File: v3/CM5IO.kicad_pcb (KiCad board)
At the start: 4 copper layers, 72 x 58 mm, 44 parts, among them J1 TYPE-C-31-M-12, J2 Conn_01x22_Female, J3 Conn_01x22_Female, J5 Conn_01x02, J6 UART Connection, J7 Micro_SD_Card_Det, J8 10164227-1001A1RLF, J9 10164227-1001A1RLF, Q1 AO3400A, SW1 Right angle Tact button, SW2 Right angle Tact button, U1 LSM9DS1, U2 74LVC1G07SE-7, U3 ASM330LHHTR, U4 XIAO_RM3100_Breakout, U5 RT9742GGJ5

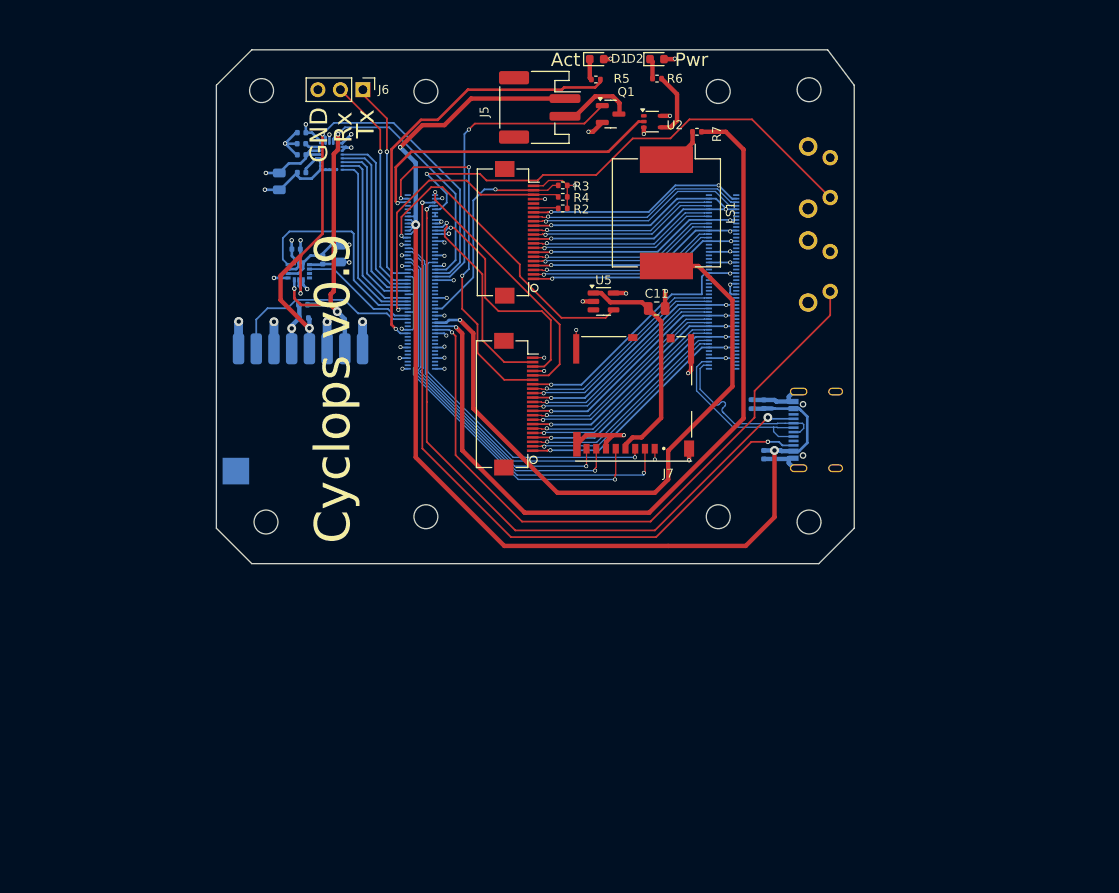
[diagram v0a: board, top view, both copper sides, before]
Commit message: Finalise v1.0 design
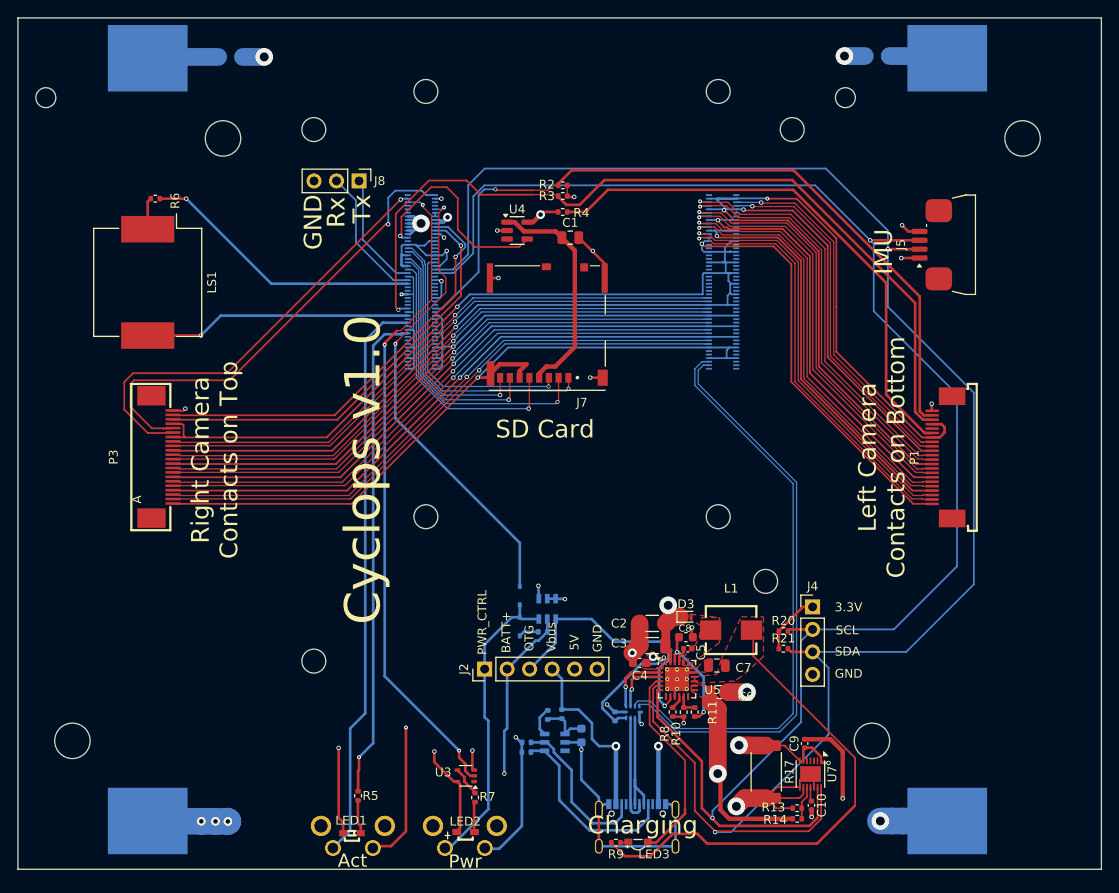
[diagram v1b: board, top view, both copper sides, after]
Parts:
- removed the C1 at (180.3, 111.7)
- removed D1: LED Green, LED_SMD:LED_0603_1608Metric
- removed D2: LED Red, LED_SMD:LED_0603_1608Metric
- removed the J3 at (152.4, 92.3)
- removed Q1: AO3400A, Package_TO_SOT_SMD:SOT-23
- removed the R4 at (157.6, 88.3)
- removed SW1, SW2: Right angle Tact button, Button_Switch_THT:SW_Tactile_SPST_Angled_PTS645Vx58-2LFS
- removed the U1 at (131.5, 83.7)
- removed the U3 at (127.8, 96.7)
- removed the U4 at (128.1, 112.2)
- added B1: BH-21700-B1BJ001, footprint:BAT-SMD_L82.5.5-W25-BH-21700-B1BJ001, B.Cu at (110.8, 115.7)
- added B2: BH-21700-B1BJ001, footprint:BAT-SMD_L82.5.5-W25-BH-21700-B1BJ001, B.Cu at (201.0, 115.7)
- added C11: 1uF, Capacitor_SMD:C_0603_1608Metric, B.Cu at (159.7, 149.1)
- added D3: NSR10F20NXT5G, Diode_SMD:Nexperia_DSN1608-2_1.6x0.8mm, F.Cu at (171.5, 135.7)
- added D5: D_Schottky, Diode_SMD:D_SOD-323, B.Cu at (152.8, 133.3)
- added D6: D_Schottky, Diode_SMD:D_SOD-323, B.Cu at (152.8, 136.8)
- added F1: Fuse, Fuse:Fuse_1206_3216Metric, B.Cu at (120.1, 72.5)
- added F2: Fuse, Fuse:Fuse_1206_3216Metric, B.Cu at (193.1, 72.4)
- added J4: Conn_01x04_Pin, Connector_PinHeader_2.54mm:PinHeader_1x04_P2.54mm_Vertical, F.Cu at (185.8, 134.6)
- added L1: MHCI05018-1R0M-R8A, footprint:IND-SMD_L5.7-W5.4, F.Cu at (176.6, 137.2)
- added LED1: MHS171CYCT, footprint:LED-SMD_L2.0-W1.1-R-RD-SIDE_YELLOW, F.Cu at (133.8, 160.1)
- added LED2: MHS171UGCT, footprint:LED-SMD_L2.0-W1.1_RD_GREEN_SIDE, F.Cu at (146.6, 160.0)
- added LED3: MHS171UBCT, footprint:LED-SMD_L2.1-W1.0-R-RD, F.Cu at (166.1, 161.1)
- added P1: AFC07-S22FCC-00 (Bottom contact), footprint:FPC-SMD_AFC07-S22FCC-00, F.Cu at (200.4, 117.7)
- added P3: FPC_0_5MM_22P_Pull_type_H2_0mm_Pick_up, footprint:FPC-SMD_P0.50-22P_LSSJ-H2.0-22P, F.Cu at (112.4, 117.7)
- added R10: 10k, Resistor_SMD:R_0402_1005Metric, F.Cu at (172.5, 146.4)
- added R11: 10k, Resistor_SMD:R_0402_1005Metric, F.Cu at (171.2, 146.5)
- added R12: 10k, Resistor_SMD:R_0402_1005Metric, B.Cu at (155.3, 137.4)
- added R13: 300k, Resistor_SMD:R_0402_1005Metric, F.Cu at (184.1, 158.5)
- added R14: 200k, Resistor_SMD:R_0402_1005Metric, F.Cu at (184.1, 157.3)
- added R15: 10k, Resistor_SMD:R_0402_1005Metric, B.Cu at (155.9, 146.8)
- added R16: 1k, Resistor_SMD:R_0402_1005Metric, B.Cu at (157.5, 146.7)
- added R17: 10mOhm, Resistor_SMD:R_2512_6332Metric, F.Cu at (180.6, 153.2)
- added R18: 5.1k, Resistor_SMD:R_0402_1005Metric, B.Cu at (153.5, 149.9)
- added R19: 5.1k, Resistor_SMD:R_0402_1005Metric, B.Cu at (153.5, 151.0)
- added R2: 2.2K 1%, Resistor_SMD:R_0402_1005Metric, F.Cu at (157.6, 87.0)
- added R20: 2.2K 1%, Resistor_SMD:R_0402_1005Metric, F.Cu at (182.5, 137.3)
- added R21: 2.2K 1%, Resistor_SMD:R_0402_1005Metric, F.Cu at (182.5, 139.3)
- added U10: TS-1093C-A5B3-D1, footprint:SW-TH_TS-1093C-A5B3-D1, B.Cu at (146.6, 160.5)
- added U2: TS3USB221ARSER, footprint:UQFN-10_L2.0-W1.5-P0.50-BL, B.Cu at (165.5, 146.4)
- added U5: BQ25895RTW, Package_DFN_QFN:Texas_RTW_WQFN-24-1EP_4x4mm_P0.5mm_EP2.7x2.7mm_ThermalVias, F.Cu at (170.5, 142.7)
- added U6: SN74LVC1G57DBVR, footprint:SOT-23-6_L2.9-W1.6-P0.95-LS2.8-BL, B.Cu at (155.8, 134.8)
- added U7: MAX17261xxTD, Package_DFN_QFN:TDFN-14-1EP_3x3mm_P0.4mm_EP1.78x2.35mm, F.Cu at (185.6, 153.4)
- added U8: CH221K, footprint:SOT-23-6_L2.9-W1.6-P0.95-LS2.8-BL-2, B.Cu at (156.7, 149.9)
- added U9: TS-1093C-A14B3-D1, footprint:SW-TH_TS-1093C-A14B3-D1, B.Cu at (133.9, 160.5)
- C1: renamed from C11; value 10u -> 10uF
- C10: value 10u -> 470nF; footprint Capacitor_SMD:C_0805_2012Metric -> Capacitor_SMD:C_0402_1005Metric; moved to F.Cu
- C2: value 100n -> 33uF; footprint Capacitor_SMD:C_0402_1005Metric -> Capacitor_SMD:C_1206_3216Metric; moved to F.Cu
- C3: value 10n -> 33uF; footprint Capacitor_SMD:C_0402_1005Metric -> Capacitor_SMD:C_1206_3216Metric; moved to F.Cu
- C4: value 100n -> 1uF; footprint Capacitor_SMD:C_0402_1005Metric -> Capacitor_SMD:C_0603_1608Metric; moved to F.Cu
- C5: value 100n -> 47nF; moved to F.Cu
- C6: value 10u -> 22uF; moved to F.Cu
- C7: value 100n -> 10uF; footprint Capacitor_SMD:C_0402_1005Metric -> Capacitor_SMD:C_0805_2012Metric; moved to F.Cu
- C8: value 100n -> 4.7uF; footprint Capacitor_SMD:C_0402_1005Metric -> Capacitor_SMD:C_0603_1608Metric; moved to F.Cu
- C9: value 100n -> 100nF; moved to F.Cu
- J2: value Conn_01x22_Female -> Conn_01x06_Pin; footprint CM5IO:Hirose_FH12-22S-0.5SH_1x22-1MP_P0.50mm_Horizontal -> Connector_PinHeader_2.54mm:PinHeader_1x06_P2.54mm_Vertical
- J5: value Conn_01x02 -> Conn_01x04_Pin; footprint Connector_JST:JST_PH_S2B-PH-SM4-TB_1x02-1MP_P2.00mm_Horizontal -> Connector_FFC-FPC:JUSHUO_AFA07-S04FCA-00_1x4-1MP_P1.0mm_Horizontal
- R1: value 2.2K 1% -> 10k
- R8: value 2.2K 1% -> 261; moved to F.Cu
- R9: value 2.2K 1% -> 2.2k 1%; moved to F.Cu
- moved H3 85.4 mm to (129.5, 140.7)
- moved R5 85.2 mm to (134.5, 155.9), turned to 90 degrees
- moved R7 83.7 mm to (147.7, 156.1), turned to 90 degrees
- moved C10 82.0 mm to (185.7, 157.0), turned to -90 degrees
- moved C9 80.1 mm to (184.9, 150.0), turned to 90 degrees
- moved C7 76.8 mm to (175.2, 144.2), turned to 0 degrees
- moved U3 76.8 mm to (146.7, 153.7), turned to 180 degrees
- moved C6 73.7 mm to (175.0, 141.2), turned to 180 degrees
- moved C5 72.8 mm to (171.7, 139.3)
- moved C4 70.0 mm to (166.3, 140.9)
- moved R9 68.9 mm to (163.6, 161.2)
- moved C3 66.5 mm to (167.7, 138.9)
- moved R8 62.1 mm to (170.0, 146.4), turned to 90 degrees
- moved R6 61.6 mm to (111.6, 88.5)
- moved H1 60.1 mm to (183.5, 80.7)
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- renumbered J8 to J3, J9 to J6, J6 to J8, R2 to R4, R7 to R6, R6 to R7, U6 to U1, U2 to U3, U5 to U4
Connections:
- C10 pad 1: /+3.3v -> Net-(U7-REG)
- C10 pad 2: GND -> -BATT
- C2 pad 1: /+5v -> /CM5_5V
- C3 pad 1: Net-(U1-CAP) -> /CM5_5V
- C4 pad 1: Net-(U1-C1) -> /Vbus
- C5 pad 1: /+3.3v -> /Power/SW
- C5 pad 2: GND -> Net-(U5-BTST)
- C6 pad 1: /+3.3v -> Vsys
- C7 pad 1: /+3.3v -> +BATT
- C8 pad 1: /+3.3v -> Net-(U5-REGN)
- C9 pad 1: /+3.3v -> +BATT
- C9 pad 2: GND -> -BATT
- J1 pad A4_B9: /+5v -> /Vbus
- J1 pad B4_A9: /+5v -> /Vbus
- J2 pad 1: GND -> /Power/PWR_CTRL
- J2 pad 2: /CM5_HighSpeed/DPHY0_D0_N -> +BATT
- J2 pad 3: /CM5_HighSpeed/DPHY0_D0_P -> /Power/OTG
- J2 pad 4: GND -> /Vbus
- J2 pad 5: /CM5_HighSpeed/DPHY0_D1_N -> /CM5_5V
- J2 pad 6: /CM5_HighSpeed/DPHY0_D1_P -> GND
- J3 pad 1: /CM5_HighSpeed/USBOTG_ID -> unconnected-(J3-USB_OTG_ID-Pad1)
- J3 pad 100: /CM5_HighSpeed/HDMI0_SCL -> unconnected-(J3-HDMI0_SCL-Pad100)
- J3 pad 11: /CM5_HighSpeed/VBUS_EN -> unconnected-(J3-VBUS_EN-Pad11)
- J3 pad 28: /CM5_HighSpeed/USB3-0-RX_N -> unconnected-(J3-USB3-0-RX_N-Pad28)
- J3 pad 3: /USB2_N -> /CM5_USB2_N
- J3 pad 30: /CM5_HighSpeed/USB3-0-RX_P -> unconnected-(J3-USB3-0-RX_P-Pad30)
- J3 pad 34: /CM5_HighSpeed/USB3-0-D_P -> unconnected-(J3-USB3-0-D_P-Pad34)
- J3 pad 36: /CM5_HighSpeed/USB3-0-D_N -> unconnected-(J3-USB3-0-D_N-Pad36)
- J3 pad 40: /CM5_HighSpeed/USB3-0-TX_N -> unconnected-(J3-USB3-0-TX_N-Pad40)
- J3 pad 42: /CM5_HighSpeed/USB3-0-TX_P -> unconnected-(J3-USB3-0-TX_P-Pad42)
- J3 pad 43: /CM5_HighSpeed/HDMI1_HOTPLUG -> unconnected-(J3-HDMI1_HOTPLUG-Pad43)
- J3 pad 45: /CM5_HighSpeed/HDMI1_SDA -> unconnected-(J3-HDMI1_SDA-Pad45)
- J3 pad 46: /CM5_HighSpeed/HDMI1_D2_P -> unconnected-(J3-HDMI1_TX2_P-Pad46)
- J3 pad 47: /CM5_HighSpeed/HDMI1_SCL -> unconnected-(J3-HDMI1_SCL-Pad47)
- J3 pad 48: /CM5_HighSpeed/HDMI1_D2_N -> unconnected-(J3-HDMI1_TX2_N-Pad48)
- J3 pad 49: /CM5_HighSpeed/HDMI1_CEC -> unconnected-(J3-HDMI1_CEC-Pad49)
- J3 pad 5: /USB2_P -> /CM5_USB2_P
- J3 pad 51: /CM5_HighSpeed/HDMI0_CEC -> unconnected-(J3-HDMI0_CEC-Pad51)
- J3 pad 52: /CM5_HighSpeed/HDMI1_D1_P -> unconnected-(J3-HDMI1_TX1_P-Pad52)
- J3 pad 53: /CM5_HighSpeed/HDMI0_HOTPLUG -> unconnected-(J3-HDMI0_HOTPLUG-Pad53)
- J3 pad 54: /CM5_HighSpeed/HDMI1_D1_N -> unconnected-(J3-HDMI1_TX1_N-Pad54)
- J3 pad 57: /CM5_HighSpeed/USB3-1-RX_N -> unconnected-(J3-USB3-1-RX_N-Pad57)
- J3 pad 58: /CM5_HighSpeed/HDMI1_D0_P -> unconnected-(J3-HDMI1_TX0_P-Pad58)
- J3 pad 59: /CM5_HighSpeed/USB3-1-RX_P -> unconnected-(J3-USB3-1-RX_P-Pad59)
- J3 pad 60: /CM5_HighSpeed/HDMI1_D0_N -> unconnected-(J3-HDMI1_TX0_N-Pad60)
- J3 pad 63: /CM5_HighSpeed/USB3-1-D_P -> unconnected-(J3-USB3-1-D_P-Pad63)
- J3 pad 64: /CM5_HighSpeed/HDMI1_CK_P -> unconnected-(J3-HDMI1_CLK_P-Pad64)
- J3 pad 65: /CM5_HighSpeed/USB3-1-D_N -> unconnected-(J3-USB3-1-D_N-Pad65)
- J3 pad 66: /CM5_HighSpeed/HDMI1_CK_N -> unconnected-(J3-HDMI1_CLK_N-Pad66)
- J3 pad 69: /CM5_HighSpeed/USB3-1-TX_N -> unconnected-(J3-USB3-1-TX_N-Pad69)
- J3 pad 70: /CM5_HighSpeed/HDMI0_D2_P -> unconnected-(J3-HDMI0_TX2_P-Pad70)
- J3 pad 71: /CM5_HighSpeed/USB3-1-TX_P -> unconnected-(J3-USB3-1-TX_P-Pad71)
- J3 pad 72: /CM5_HighSpeed/HDMI0_D2_N -> unconnected-(J3-HDMI0_TX2_N-Pad72)
- J3 pad 76: /CM5_HighSpeed/HDMI0_D1_P -> unconnected-(J3-HDMI0_TX1_P-Pad76)
- J3 pad 78: /CM5_HighSpeed/HDMI0_D1_N -> unconnected-(J3-HDMI0_TX1_N-Pad78)
- J3 pad 82: /CM5_HighSpeed/HDMI0_D0_P -> unconnected-(J3-HDMI0_TX0_P-Pad82)
- J3 pad 84: /CM5_HighSpeed/HDMI0_D0_N -> unconnected-(J3-HDMI0_TX0_N-Pad84)
- J3 pad 88: /CM5_HighSpeed/HDMI0_CK_P -> unconnected-(J3-HDMI0_CLK_P-Pad88)
- J3 pad 90: /CM5_HighSpeed/HDMI0_CK_N -> unconnected-(J3-HDMI0_CLK_N-Pad90)
- J3 pad 99: /CM5_HighSpeed/HDMI0_SDA -> unconnected-(J3-HDMI0_SDA-Pad99)
- J5 pad 1: /+5v -> GND
- J5 pad 2: Net-(J5-Pin_2) -> /PWR_SDA
- J6 pad 10: /CM5_GPIO ( Ethernet, GPIO, SDCARD)/TRD0_N -> unconnected-(J6-Ethernet_Pair0_N-Pad10)
- J6 pad 11: /CM5_GPIO ( Ethernet, GPIO, SDCARD)/TRD2_P -> unconnected-(J6-Ethernet_Pair2_P-Pad11)
- J6 pad 12: /CM5_GPIO ( Ethernet, GPIO, SDCARD)/TRD0_P -> unconnected-(J6-Ethernet_Pair0_P-Pad12)
- J6 pad 15: /CM5_GPIO ( Ethernet, GPIO, SDCARD)/ETH_LEDY -> unconnected-(J6-Ethernet_nLED3(3.3v)-Pad15)
- J6 pad 16: /CM5_GPIO ( Ethernet, GPIO, SDCARD)/TACHO -> unconnected-(J6-FAN_TACHO-Pad16)
- J6 pad 17: /CM5_GPIO ( Ethernet, GPIO, SDCARD)/ETH_LEDG -> unconnected-(J6-Ethernet_nLED2(3.3v)-Pad17)
- J6 pad 18: /CM5_GPIO ( Ethernet, GPIO, SDCARD)/SYNC_OUT -> unconnected-(J6-Ethernet_SYNC_OUT(3.3v)-Pad18)
- J6 pad 19: /CM5_GPIO ( Ethernet, GPIO, SDCARD)/PWM -> unconnected-(J6-FAN_PWM-Pad19)
- J6 pad 20: /CM5_GPIO ( Ethernet, GPIO, SDCARD)/EEPROM_nWP -> unconnected-(J6-EEPROM_nWP-Pad20)
- J6 pad 24: /CM5_GPIO ( Ethernet, GPIO, SDCARD)/GPIO26 -> unconnected-(J6-GPIO26-Pad24)
- J6 pad 25: /CM5_GPIO ( Ethernet, GPIO, SDCARD)/GPIO21 -> unconnected-(J6-GPIO21-Pad25)
- J6 pad 26: /CM5_GPIO ( Ethernet, GPIO, SDCARD)/GPIO19 -> unconnected-(J6-GPIO19-Pad26)
- J6 pad 27: /CM5_GPIO ( Ethernet, GPIO, SDCARD)/GPIO20 -> /CM5_GPIO ( Ethernet, GPIO, SDCARD)/BUTTON
- J6 pad 28: /CM5_GPIO ( Ethernet, GPIO, SDCARD)/GPIO13 -> unconnected-(J6-GPIO13-Pad28)
- J6 pad 29: /CM5_GPIO ( Ethernet, GPIO, SDCARD)/GPIO16 -> unconnected-(J6-GPIO16-Pad29)
- J6 pad 3: /CM5_GPIO ( Ethernet, GPIO, SDCARD)/TRD3_P -> unconnected-(J6-Ethernet_Pair3_P-Pad3)
- J6 pad 30: /CM5_GPIO ( Ethernet, GPIO, SDCARD)/GPIO6 -> unconnected-(J6-GPIO6-Pad30)
- J6 pad 31: /CM5_GPIO ( Ethernet, GPIO, SDCARD)/GPIO12 -> /CM5_GPIO ( Ethernet, GPIO, SDCARD)/BUZZ_B
- J6 pad 34: /CM5_GPIO ( Ethernet, GPIO, SDCARD)/GPIO5 -> unconnected-(J6-GPIO5-Pad34)
- J6 pad 37: /CM5_GPIO ( Ethernet, GPIO, SDCARD)/GPIO7 -> unconnected-(J6-GPIO7-Pad37)
- J6 pad 38: /CM5_GPIO ( Ethernet, GPIO, SDCARD)/GPIO11 -> unconnected-(J6-GPIO11-Pad38)
- J6 pad 39: /CM5_GPIO ( Ethernet, GPIO, SDCARD)/GPIO8 -> unconnected-(J6-GPIO8-Pad39)
- J6 pad 4: /CM5_GPIO ( Ethernet, GPIO, SDCARD)/TRD1_P -> unconnected-(J6-Ethernet_Pair1_P-Pad4)
- J6 pad 40: /CM5_GPIO ( Ethernet, GPIO, SDCARD)/GPIO9 -> unconnected-(J6-GPIO9-Pad40)
- J6 pad 41: /CM5_GPIO ( Ethernet, GPIO, SDCARD)/GPIO25 -> unconnected-(J6-GPIO25-Pad41)
- J6 pad 44: /CM5_GPIO ( Ethernet, GPIO, SDCARD)/GPIO10 -> unconnected-(J6-GPIO10-Pad44)
- J6 pad 45: /CM5_GPIO ( Ethernet, GPIO, SDCARD)/GPIO24 -> unconnected-(J6-GPIO24-Pad45)
- J6 pad 46: /CM5_GPIO ( Ethernet, GPIO, SDCARD)/GPIO22 -> unconnected-(J6-GPIO22-Pad46)
- J6 pad 47: /CM5_GPIO ( Ethernet, GPIO, SDCARD)/GPIO23 -> unconnected-(J6-GPIO23-Pad47)
- J6 pad 48: /CM5_GPIO ( Ethernet, GPIO, SDCARD)/GPIO27 -> unconnected-(J6-GPIO27-Pad48)
- J6 pad 49: /CM5_GPIO ( Ethernet, GPIO, SDCARD)/GPIO18 -> /CM5_GPIO ( Ethernet, GPIO, SDCARD)/BUZZ_A
- J6 pad 5: /CM5_GPIO ( Ethernet, GPIO, SDCARD)/TRD3_N -> unconnected-(J6-Ethernet_Pair3_N-Pad5)
- J6 pad 50: /CM5_GPIO ( Ethernet, GPIO, SDCARD)/GPIO17 -> unconnected-(J6-GPIO17-Pad50)
- J6 pad 54: /CM5_GPIO ( Ethernet, GPIO, SDCARD)/GPIO4 -> unconnected-(J6-GPIO4-Pad54)
- J6 pad 56: /CM5_GPIO ( Ethernet, GPIO, SDCARD)/GPIO3 -> /PWR_SCL
- J6 pad 58: /CM5_GPIO ( Ethernet, GPIO, SDCARD)/GPIO2 -> /PWR_SDA
- J6 pad 6: /CM5_GPIO ( Ethernet, GPIO, SDCARD)/TRD1_N -> unconnected-(J6-Ethernet_Pair1_N-Pad6)
- J6 pad 76: /CM5_GPIO ( Ethernet, GPIO, SDCARD)/VBAT -> unconnected-(J6-VBAT-Pad76)
- J6 pad 77: /+5v -> /CM5_5V
- J6 pad 79: /+5v -> /CM5_5V
- J6 pad 81: /+5v -> /CM5_5V
- J6 pad 83: /+5v -> /CM5_5V
- J6 pad 85: /+5v -> /CM5_5V
- J6 pad 87: /+5v -> /CM5_5V
- J6 pad 89: /CM5_GPIO ( Ethernet, GPIO, SDCARD)/WL_nDis -> unconnected-(J6-WiFi_nDisable-Pad89)
- J6 pad 9: /CM5_GPIO ( Ethernet, GPIO, SDCARD)/TRD2_N -> unconnected-(J6-Ethernet_Pair2_N-Pad9)
- J6 pad 91: /CM5_GPIO ( Ethernet, GPIO, SDCARD)/BT_nDis -> unconnected-(J6-BT_nDisable-Pad91)
- J6 pad 92: /CM5_GPIO ( Ethernet, GPIO, SDCARD)/PWR_BUT -> /PWR_BUT
- J6 pad 93: /CM5_GPIO ( Ethernet, GPIO, SDCARD)/nRPIBOOT -> unconnected-(J6-nRPIBOOT-Pad93)
- J6 pad 94: /CC1 -> unconnected-(J6-CC1-Pad94)
- J6 pad 96: /CC2 -> unconnected-(J6-CC2-Pad96)
- J6 pad 99: /CM5_GPIO ( Ethernet, GPIO, SDCARD)/PMIC_ENABLE -> unconnected-(J6-PMIC_ENABLE-Pad99)
- LS1 pad 2: /CM5_GPIO ( Ethernet, GPIO, SDCARD)/GPIO13 -> /CM5_GPIO ( Ethernet, GPIO, SDCARD)/BUZZ_B
- R1 pad 1: /+5v -> /+3.3v
- R1 pad 2: GND -> /DSEL
- R3 pad 2: /CM5_GPIO ( Ethernet, GPIO, SDCARD)/ID_SD -> /CM5_GPIO ( Ethernet, GPIO, SDCARD)/ID_SC
- R6 pad 1: /CM5_GPIO ( Ethernet, GPIO, SDCARD)/GPIO19 -> /CM5_GPIO ( Ethernet, GPIO, SDCARD)/BUZZ_A
- R8 pad 1: /+3.3v -> GND
- R8 pad 2: /CM5_GPIO ( Ethernet, GPIO, SDCARD)/GPIO2 -> Net-(U5-ILIM)
- R9 pad 1: /+3.3v -> Vsys
- R9 pad 2: /CM5_GPIO ( Ethernet, GPIO, SDCARD)/GPIO3 -> Net-(LED3-A)
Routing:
- net GND: track 425.4 -> 883.2 mm, vias 63 -> 32
- net +BATT: track 0.00 -> 322.7 mm, vias 0 -> 5
- net /PWR_SDA: track 0.00 -> 198.5 mm, vias 0 -> 2
- net /PWR_SCL: track 0.00 -> 187.3 mm, vias 0 -> 2
- net /+5v: track 131.3 -> 0.00 mm, vias 3 -> 0
- net /CM5_GPIO ( Ethernet, GPIO, SDCARD)/GPIO19: track 91.6 -> 0.00 mm, vias 1 -> 0
- net /CM5_5V: track 0.00 -> 84.6 mm, vias 0 -> 2
- net /CM5_GPIO ( Ethernet, GPIO, SDCARD)/GPIO26: track 75.5 -> 0.00 mm, vias 1 -> 0
- net /CM5_GPIO ( Ethernet, GPIO, SDCARD)/GPIO13: track 72.4 -> 0.00 mm, vias 1 -> 0
- net /CM5_GPIO ( Ethernet, GPIO, SDCARD)/GPIO3: track 66.5 -> 0.00 mm, vias 3 -> 0
- net /CM5_USB2_P: track 0.00 -> 65.6 mm
- net /CM5_USB2_N: track 0.00 -> 65.0 mm
- net /CM5_GPIO ( Ethernet, GPIO, SDCARD)/BUTTON: track 0.00 -> 64.4 mm
- net /CM5_GPIO ( Ethernet, GPIO, SDCARD)/GPIO2: track 63.6 -> 0.00 mm, vias 3 -> 0
- net /CM5_GPIO ( Ethernet, GPIO, SDCARD)/ID_SC: track 32.7 -> 94.9 mm
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- added copper zone on F.Cu, net +BATT
- added copper zone on In2.Cu, net -BATT
- added copper zone on F.Cu, net /Power/SW
- added copper zone on F.Cu, net /Vbus
- added copper zone on F.Cu, net GND
- added copper zone on F.Cu, net Vsys
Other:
- board size 72 x 58 mm -> 122.3 x 96.1 mm
- board text added: "3.3V"
- board text added: "5V"
- board text added: "BATT+"
- board text added: "Charging"
- board text added: "Cyclops v1.0"
- board text added: "IMU"
- board text added: "Left Camera Contacts on Bottom"
- board text added: "OTG"
- board text added: "PWR_CTRL"
- board text added: "Right Camera Contacts on Top"
- board text added: "SCL"
- board text added: "SD Card"
- board text added: "SDA"
- board text added: "Vbus"
- board text removed: "Cyclops v0.9"
